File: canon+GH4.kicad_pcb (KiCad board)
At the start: 2 copper layers, 28.5 x 35.5 mm, 16 parts, among them Q1 2SC1815, Q2 2SC1815, Q3 2SC1815

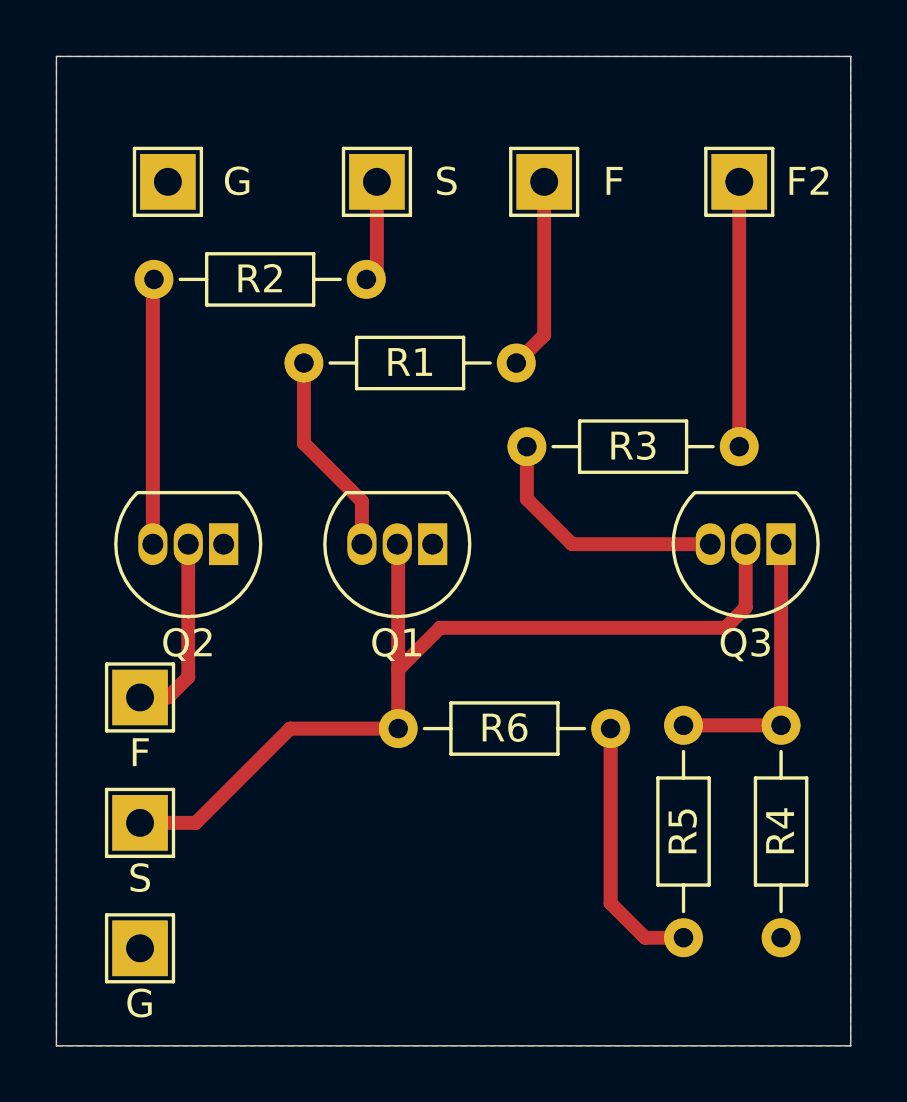
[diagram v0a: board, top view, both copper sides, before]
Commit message: updates
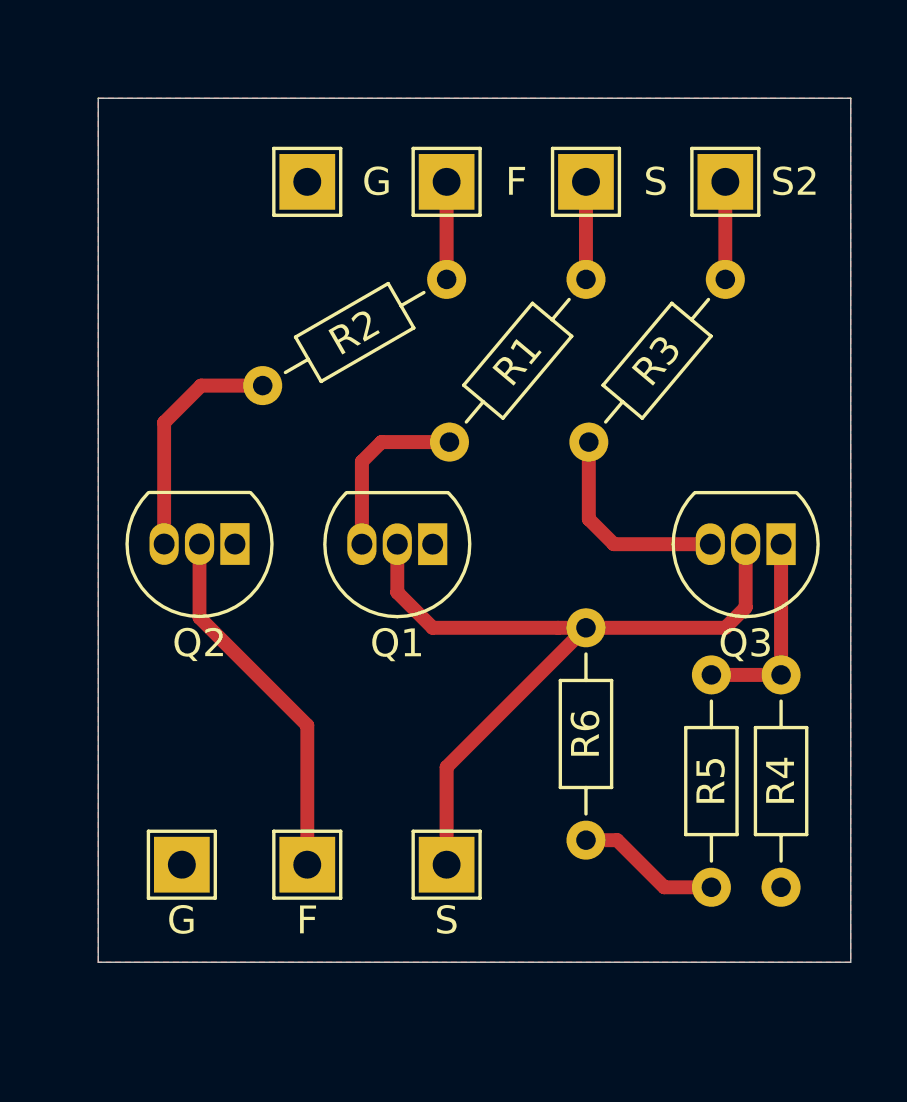
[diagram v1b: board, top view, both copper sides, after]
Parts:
- TP5: value F -> S
- TP6: value S -> F
- TP7: value F2 -> S2
- moved TP2 11.1 mm to (117.5, 92.5)
- moved R5 9.48 mm to (127.0, 85.7), turned to -90 degrees
- moved R4 9.43 mm to (129.5, 85.7), turned to -90 degrees
- moved TP3 8.49 mm to (112.5, 92.5)
- moved R6 7.84 mm to (122.5, 91.6), turned to 90 degrees
- moved R3 6.02 mm to (127.5, 71.5), turned to -130 degrees
- moved TP4 5.00 mm to (112.5, 68.0)
- moved R1 3.91 mm to (122.5, 71.5), turned to -130 degrees
- moved TP1 3.35 mm to (108.0, 92.5)
- moved R2 2.88 mm to (117.5, 71.5), turned to -150 degrees
- moved TP6 2.50 mm to (117.5, 68.0)
- moved TP5 1.50 mm to (122.5, 68.0)
- moved TP7 0.50 mm to (127.5, 68.0)
- moved Q2 0.40 mm to (109.9, 81.0)
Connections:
- net /Signal_focus renamed /Focus_Input
- net /Signal_shutter renamed /Shutter_Input
- net Net-(Q2-C) renamed /Focus_Output
- net Net-(R6-Pad1) renamed /Focus_Input_GH4
- Q1 pad 1: /Ground -> GND
- Q1 pad 2: Net-(Q1-C) -> /Shutter_Output
- Q2 pad 1: /Ground -> GND
- Q3 pad 2: Net-(Q1-C) -> /Shutter_Output
- R4 pad 1: /Ground -> Net-(Q3-E)
- R4 pad 2: Net-(Q3-E) -> GND
- R5 pad 1: Net-(R4-Pad1) -> Net-(Q3-E)
- R5 pad 2: Net-(Q3-E) -> Net-(R5-Pad2)
- R6 pad 1: Net-(Q1-C) -> Net-(R5-Pad2)
- R6 pad 2: Net-(R4-Pad1) -> /Shutter_Output
- TP1 pad 1: /Ground -> GND
- TP2 pad 1: Net-(Q1-C) -> /Shutter_Output
- TP4 pad 1: /Ground -> GND
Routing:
- net Net-(Q1-C): track 33.0 -> 0.00 mm
- net /Shutter_Output: track 0.00 -> 27.9 mm
- net Net-(Q3-E): track 16.9 -> 7.19 mm
- net Net-(R4-Pad1): track 9.40 -> 0.00 mm
- net /Focus_Output: track 6.80 -> 13.1 mm
- net /Focus_Input_GH4: track 9.50 -> 3.50 mm
- net Net-(R5-Pad2): track 0.00 -> 5.20 mm
- net /Shutter_Input: track 6.91 -> 3.50 mm
- net Net-(Q3-B): track 9.13 -> 7.50 mm
- net Net-(Q2-B): track 9.52 -> 8.44 mm
- net Net-(Q1-B): track 7.36 -> 6.39 mm
- added copper zone on F.Cu, net GND
- removed copper zone on F.Cu, net /Ground
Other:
- board size 28.5 x 35.5 mm -> 27 x 31 mm
